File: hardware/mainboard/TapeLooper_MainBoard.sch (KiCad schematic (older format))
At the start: 8 parts, among them J1 Micro_SD_Card, U1 DAISY_SEED

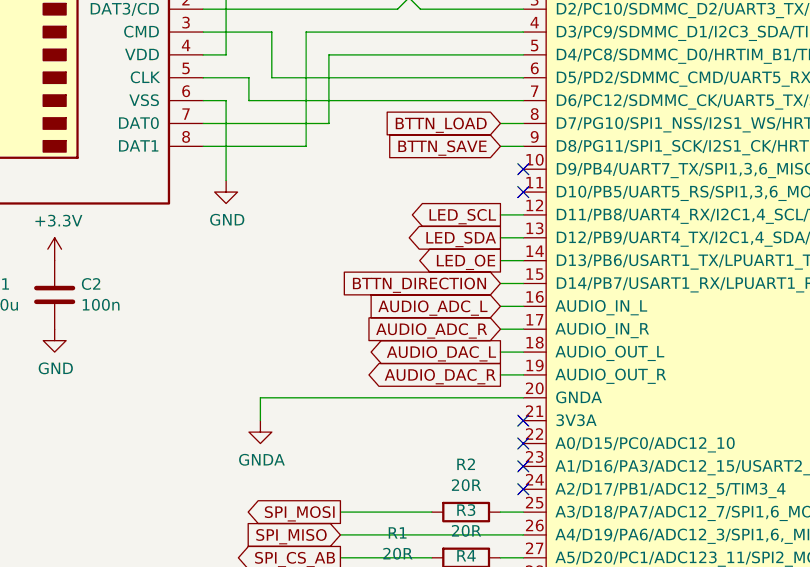
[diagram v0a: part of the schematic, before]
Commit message: hardware: update schematics & add BOM
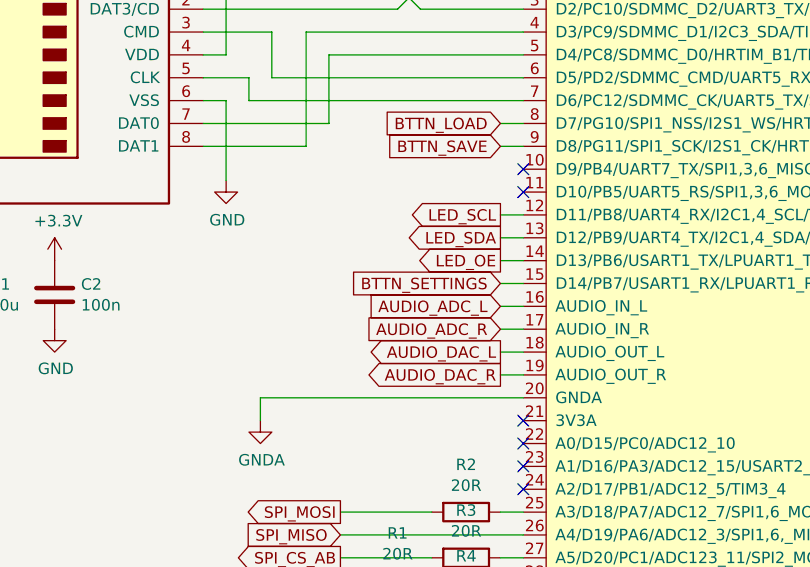
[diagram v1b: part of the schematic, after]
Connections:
- net BTTN_DIRECTION renamed BTTN_SETTINGS
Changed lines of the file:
@@
 BTTN_SAVE
 Text GLabel 7450 2600 0    50   Input ~ 0
-BTTN_DIRECTION
+BTTN_SETTINGS
 Text GLabel 7450 1200 0    50   Input ~ 0
 BTTN_REC
